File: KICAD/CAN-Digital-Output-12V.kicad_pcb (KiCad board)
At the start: 2 copper layers, 84.1 x 75.4 mm, 46 parts, among them J1 UPDI Header, J2 Conn_01x04_Female, J3 UART Header, K1 CP1SA-12V-X, K2 CP1SA-12V-X, K3 CP1SA-12V-X, K4 CP1SA-12V-X, Q1 MMBT2222A-TP, Q2 MMBT2222A-TP, Q3 MMBT2222A-TP, Q4 MMBT2222A-TP, U1 AZ1117-5.0, U2 MCP2551-I-SN, U3 ATtiny414-SS, U4 1-2834011-3, U5 MCP2515-xSO, U6 1-2834011-3, U7 1-2834011-3, U8 1-2834011-3, Y1 8MHz

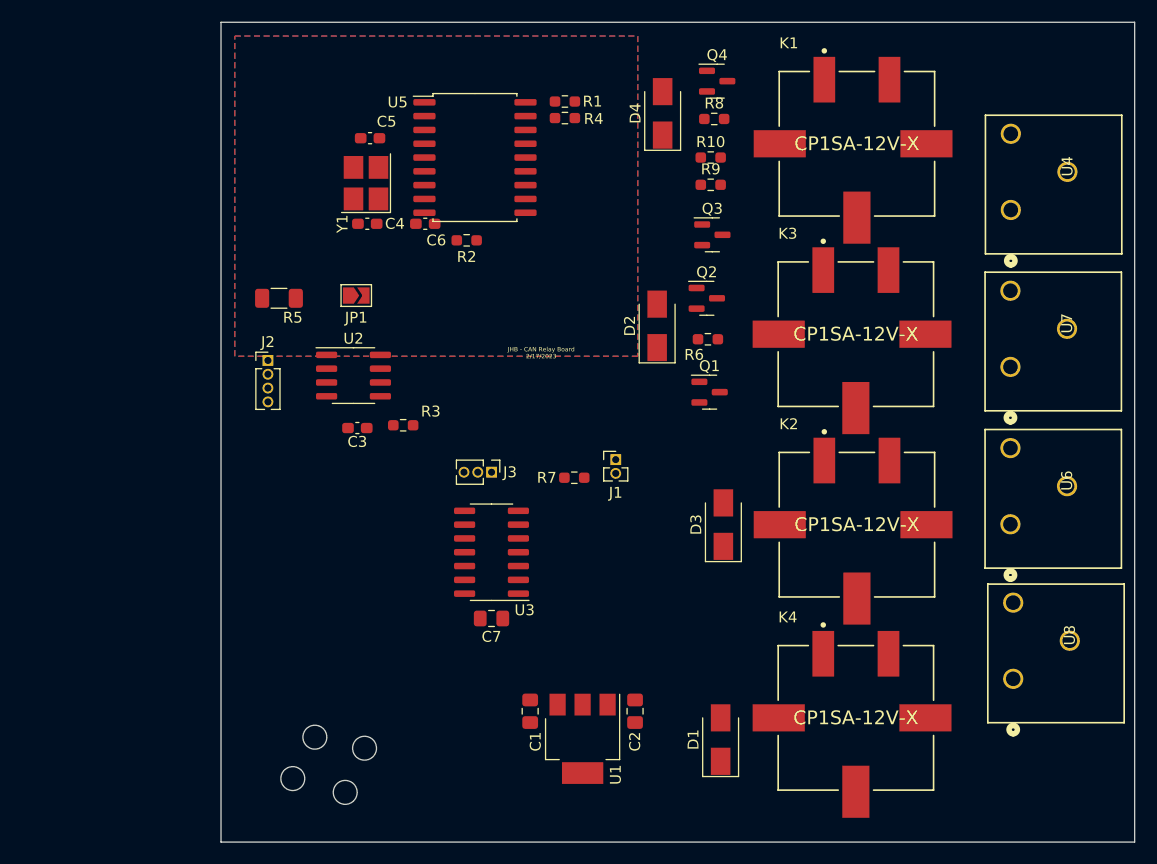
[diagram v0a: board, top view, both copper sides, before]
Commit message: Design review with Jarrod
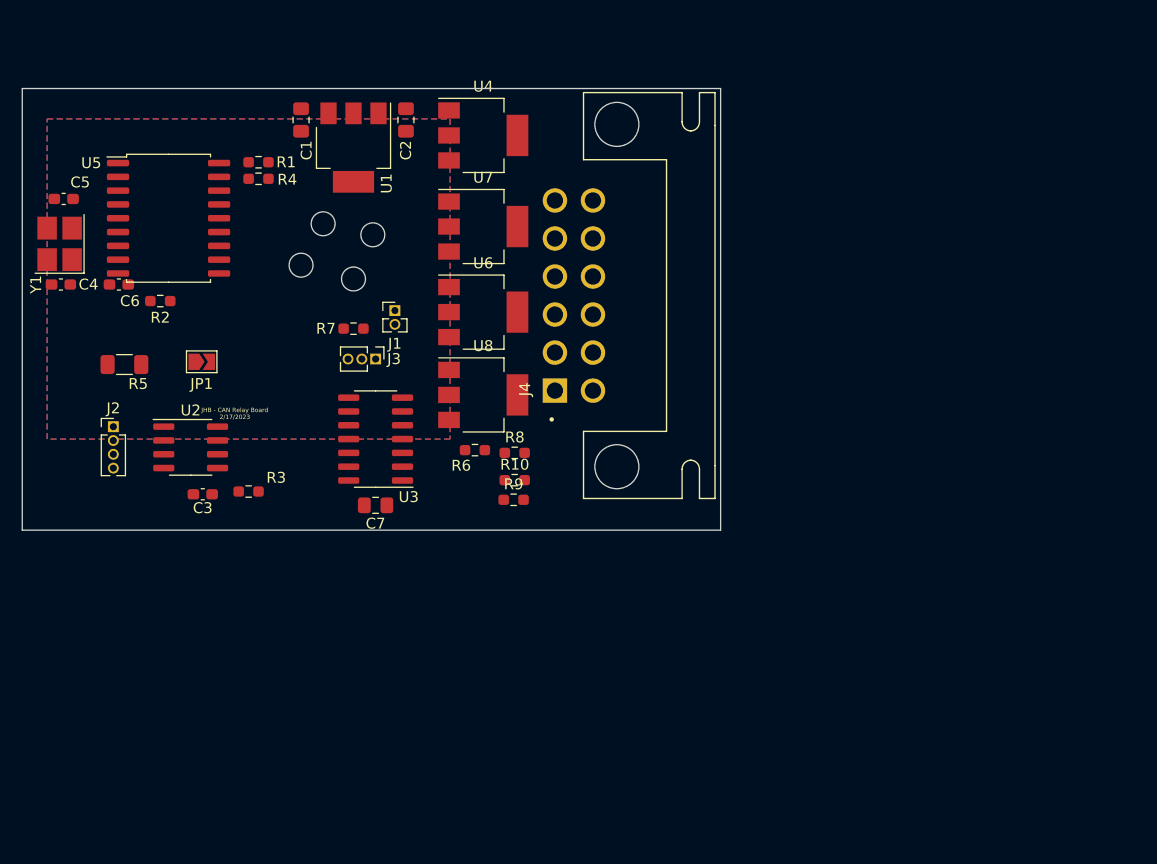
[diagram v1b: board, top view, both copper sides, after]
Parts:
- removed D1, D2, D3, D4: NRVA4007T3G, Diode_SMD:D_SMA
- removed K1, K2, K3, K4: CP1SA-12V-X, eec:Panasonic-CP1SA-12V-X-MFG
- removed Q1, Q2, Q3, Q4: MMBT2222A-TP, Package_TO_SOT_SMD:SOT-23
- added J4: 0367831201, 0367831201:MOLEX_0367831201, F.Cu at (181.2, 101.9)
- U4, U6, U7, U8: value 1-2834011-3 -> VNL5050N3TR-E; footprint 1-2834011-3:CONN_1-2834011-3 -> Package_TO_SOT_SMD:SOT-223
- moved C1 58.3 mm to (152.1, 85.7)
- moved C2 58.3 mm to (161.8, 85.7)
- moved U1 58.3 mm to (157.0, 88.2)
- moved U8 55.3 mm to (168.9, 111.0), turned to 0 degrees
- moved U6 52.3 mm to (168.9, 103.4), turned to 0 degrees
- moved U7 50.2 mm to (168.9, 95.5), turned to 0 degrees
- moved U4 49.0 mm to (168.9, 87.1), turned to 0 degrees
- moved H4 47.3 mm to (157.0, 100.3)
- moved H2 47.3 mm to (154.2, 95.2)
- moved H3 47.3 mm to (152.1, 99.1)
- moved H1 47.3 mm to (158.8, 96.3)
- moved R8 35.8 mm to (171.8, 116.3)
- moved R10 34.7 mm to (171.8, 118.8)
- moved R9 34.2 mm to (171.7, 120.7)
- moved C5 28.7 mm to (130.3, 93.0)
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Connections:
- R10 pad 1: /RELAY_1 -> /OUT_4
- R10 pad 2: Net-(Q4-Pad1) -> Net-(R10-Pad2)
- R6 pad 1: /RELAY_1 -> /OUT_1
- R6 pad 2: Net-(Q1-Pad1) -> Net-(R6-Pad2)
- R8 pad 1: /RELAY_1 -> /OUT_2
- R8 pad 2: Net-(Q2-Pad1) -> Net-(R8-Pad2)
- R9 pad 1: /RELAY_1 -> /OUT_3
- R9 pad 2: Net-(Q3-Pad1) -> Net-(R9-Pad2)
- U3 pad 2: /RELAY_2 -> /OUT_2
- U3 pad 3: /RELAY_3 -> /OUT_3
- U3 pad 5: /RELAY_4 -> /OUT_4
- U3 pad 8: /RELAY_1 -> /OUT_1
- U4 pad 1: Net-(K1-Pad3) -> Net-(R6-Pad2)
- U4 pad 2: Net-(K1-Pad5) -> /DO_1
- U4 pad 3: Net-(K1-Pad4) -> GND
- U6 pad 1: Net-(K2-Pad3) -> Net-(R8-Pad2)
- U6 pad 2: Net-(K2-Pad5) -> /DO_2
- U6 pad 3: Net-(K2-Pad4) -> GND
- U7 pad 1: Net-(K3-Pad3) -> Net-(R9-Pad2)
- U7 pad 2: Net-(K3-Pad5) -> /DO_3
- U7 pad 3: Net-(K3-Pad4) -> GND
- U8 pad 1: Net-(K4-Pad3) -> Net-(R10-Pad2)
- U8 pad 2: Net-(K4-Pad5) -> /DO_4
- U8 pad 3: Net-(K4-Pad4) -> GND
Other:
- board size 84.1 x 75.4 mm -> 64.3 x 40.6 mm

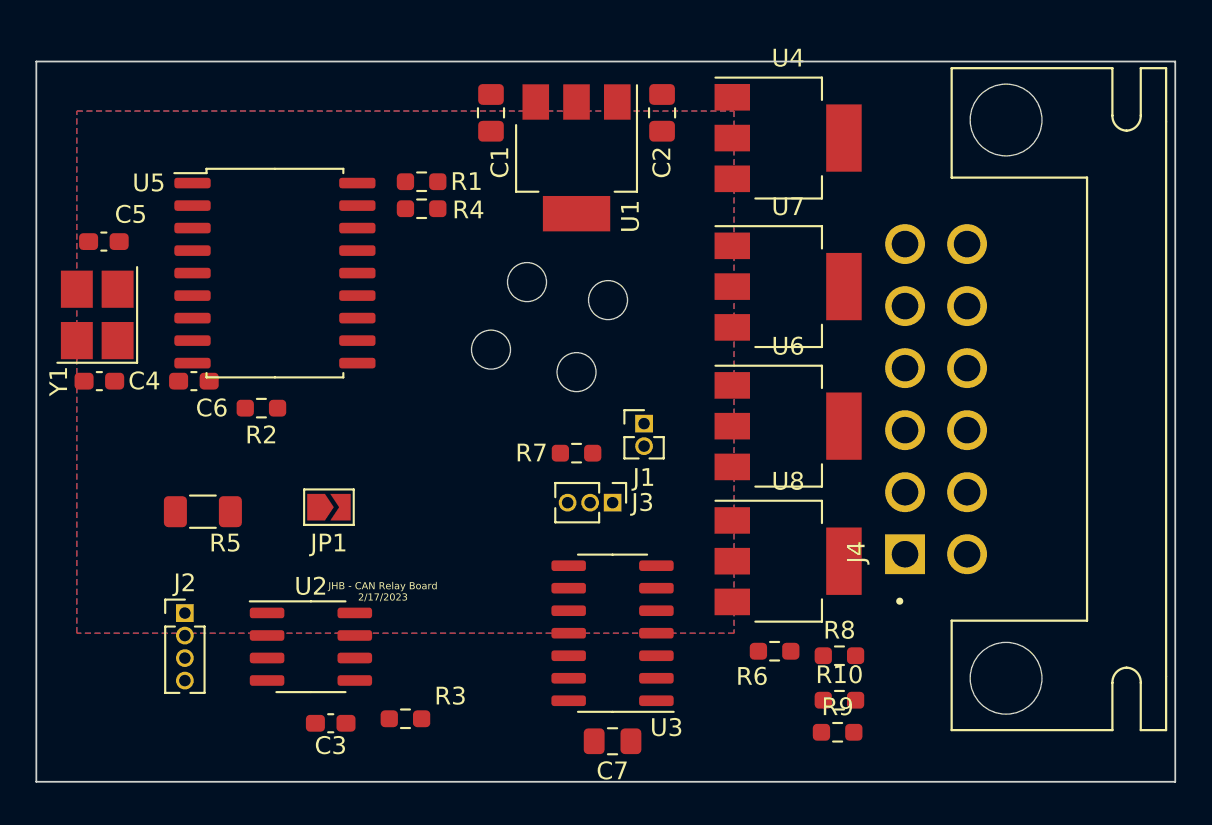
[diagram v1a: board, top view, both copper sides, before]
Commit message: Third Design Review
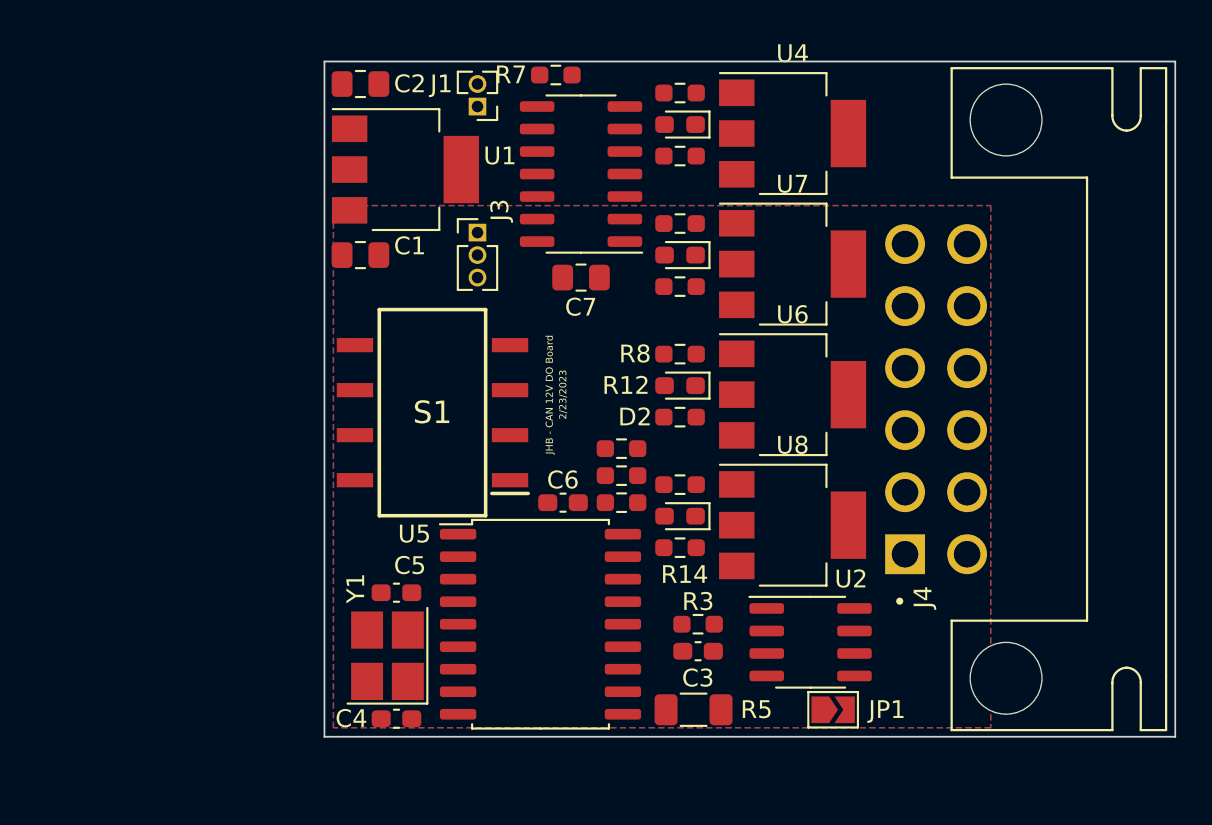
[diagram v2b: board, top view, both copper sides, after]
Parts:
- removed H1, H2, H3, H4: MountingHole, MountingHole:MountingHole_2.2mm_M2_ISO14580
- removed J2: Conn_01x04_Female, Connector_PinHeader_1.27mm:PinHeader_1x04_P1.27mm_Vertical
- added D1: LED, LED_SMD:LED_0603_1608Metric_Pad1.05x0.95mm_HandSolder, F.Cu at (162.8, 86.4)
- added D2: LED, LED_SMD:LED_0603_1608Metric_Pad1.05x0.95mm_HandSolder, F.Cu at (162.8, 101.1)
- added D3: LED, LED_SMD:LED_0603_1608Metric_Pad1.05x0.95mm_HandSolder, F.Cu at (162.8, 93.7)
- added D4: LED, LED_SMD:LED_0603_1608Metric_Pad1.05x0.95mm_HandSolder, F.Cu at (162.8, 108.5)
- added R11: 150, Resistor_SMD:R_0603_1608Metric_Pad0.98x0.95mm_HandSolder, F.Cu at (162.8, 88.1)
- added R12: 150, Resistor_SMD:R_0603_1608Metric_Pad0.98x0.95mm_HandSolder, F.Cu at (162.8, 102.9)
- added R13: 150, Resistor_SMD:R_0603_1608Metric_Pad0.98x0.95mm_HandSolder, F.Cu at (162.8, 95.5)
- added R14: 150, Resistor_SMD:R_0603_1608Metric_Pad0.98x0.95mm_HandSolder, F.Cu at (162.8, 110.2)
- added S1: 219-4MSTR, 219-4MSTR:SOP254P991X385-8N, F.Cu at (148.8, 102.6)
- moved R6 31.9 mm to (162.8, 84.6), turned to 0 degrees
- moved JP1 30.7 mm to (171.4, 119.4)
- moved R9 30.0 mm to (162.8, 91.9)
- moved R5 29.9 mm to (163.6, 119.4)
- moved U2 28.2 mm to (170.2, 115.6)
- moved C7 26.2 mm to (157.2, 95.0)
- moved U3 26.0 mm to (157.2, 89.2)
- moved C5 25.8 mm to (146.8, 112.8)
- moved C4 25.4 mm to (146.8, 119.9)
- moved Y1 25.3 mm to (146.3, 116.3)
- moved U5 24.8 mm to (154.9, 114.6)
- moved C6 21.9 mm to (156.2, 107.7)
- moved R7 21.4 mm to (155.8, 83.6), turned to 0 degrees
- moved C3 21.1 mm to (163.8, 116.1)
- moved R2 20.4 mm to (159.5, 104.6)
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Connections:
- J4 pad 1: unconnected-(J4-Pad1) -> VCC
- J4 pad 10: unconnected-(J4-Pad10) -> /DO_4
- J4 pad 11: unconnected-(J4-Pad11) -> /CAN_H
- J4 pad 12: unconnected-(J4-Pad12) -> /CAN_L
- J4 pad 2: unconnected-(J4-Pad2) -> VCC
- J4 pad 3: unconnected-(J4-Pad3) -> VCC
- J4 pad 4: unconnected-(J4-Pad4) -> GND
- J4 pad 5: unconnected-(J4-Pad5) -> GND
- J4 pad 6: unconnected-(J4-Pad6) -> GND
- J4 pad 7: unconnected-(J4-Pad7) -> /DO_1
- J4 pad 8: unconnected-(J4-Pad8) -> /DO_2
- J4 pad 9: unconnected-(J4-Pad9) -> /DO_3
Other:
- board size 64.3 x 40.6 mm -> 48 x 38.1 mm
- board text added: "2/23/2023"
- board text added: "JHB - CAN 12V DO Board"
- board text removed: "2/17/2023"
- board text removed: "JHB - CAN Relay Board"
